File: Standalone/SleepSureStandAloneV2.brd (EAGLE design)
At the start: 62.3 x 37 mm, 79 parts, among them IC1 CP2104, J1 10118192-0002LF, Q1 mmbt2222, Q2 mmbt2222, Q3 DMG3415U, SW2 KMR2, T1 MMUN2133LT1G, U1 ADS1299-4PAG, U2 AP2112-3.3, U3 MCP73831T-2ACI/OT, U4 TPS61090RSAR, X1 JSTPH, X2 ESP32_WROOM32_SKINNY

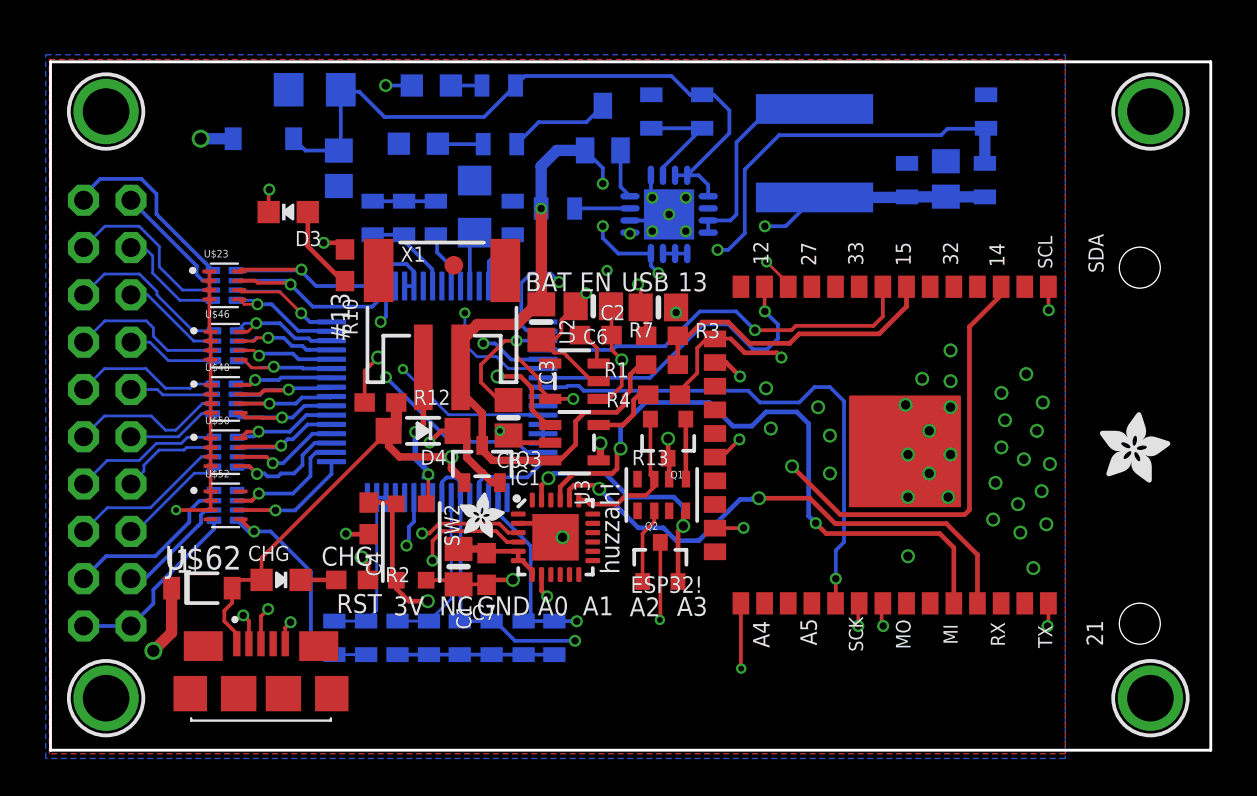
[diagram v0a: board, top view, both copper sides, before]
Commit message: Uploading final standalone and feather files
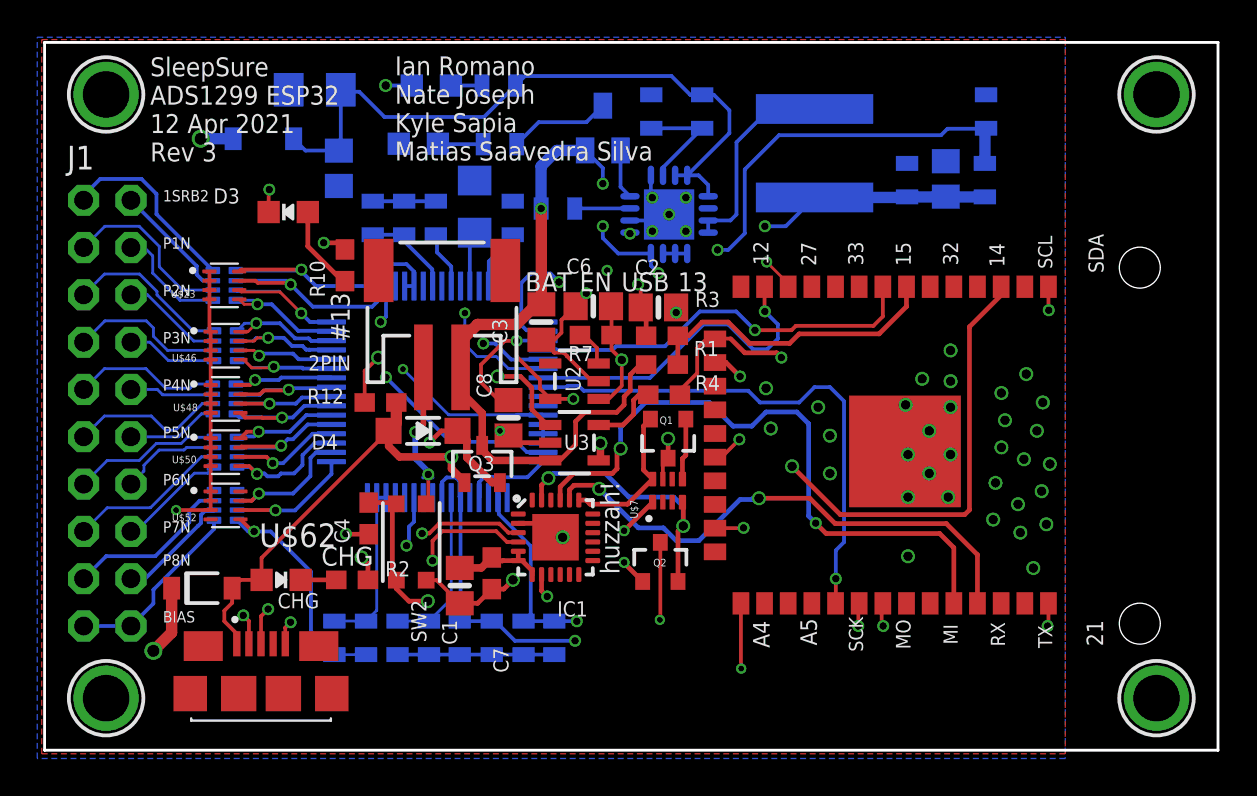
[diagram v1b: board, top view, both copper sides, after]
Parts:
- removed R13: 10K, microbuilder:RESPACK_4X0603
- removed U$14: (no value), microbuilder:ADAFRUIT_2.5MM
- removed U$15: (no value), microbuilder:ADAFRUIT_3.5MM
- removed U$34: FIDUCIAL_1MM, microbuilder:FIDUCIAL_1MM
- added U$7: 10k, SleepSureLib:RESCAXS50P200X100X45-8N
- JP2: value (none) -> 2x10
- U3: value MCP73831T-2ACI/OT -> LiPoly
- moved C1 1.02 mm to (22.3, 8.84)
- moved U$19 0.97 mm to (59.7, 35.2)
- moved U$6 0.92 mm to (3.30, 35.2)
- moved C7 0.36 mm to (24.0, 9.50)
- moved U$31 0.33 mm to (59.7, 2.79)
- renumbered X1 to 2PIN
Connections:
- removed net N$12: Q1.1, R13.5
- removed net N$13: Q2.1, R13.2
- new net N$2: Q2.1, U$7.1
- new net N$6: Q1.1, U$7.5
- net 3.3V: now also U$7.2; no longer R13.3
- net DTR: now also U$7.4; no longer R13.4
- net RESET: now also U$7.7; no longer R13.6
- net RTS: now also U$7.8; no longer R13.7
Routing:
- net N$2: track 0.00 -> 5.30 mm, vias 0 -> 2
- net N$13: track 4.06 -> 0.00 mm
- net N$6: track 0.00 -> 3.30 mm
- net N$12: track 3.23 -> 0.00 mm
- net GND: track 81.5 -> 82.7 mm
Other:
- board size 62.3 x 37 mm -> 63 x 38 mm
- board text added: "1SRB2"
- board text added: "BIAS"
- board text added: "Ian Romano Nate Joseph Kyle Sapia Matias Saavedra Silva"
- board text added: "P1N"
- board text added: "P2N"
- board text added: "P3N"
- board text added: "P4N"
- board text added: "P5N"
- board text added: "P6N"
- board text added: "P7N"
- board text added: "P8N"
- board text added: "SleepSure ADS1299 ESP32 12 Apr 2021 Rev 3"
- board text removed: "3.7/4.2V LiPoly Batt µUSB charge"
- board text removed: "3V"
- board text removed: "A0"
- board text removed: "A1"
- board text removed: "A2"
- board text removed: "A3"
- board text removed: "ESP32 Feather 16MB Flash WiFI+BT"
- board text removed: "ESP32!"
- board text removed: "GND"
- board text removed: "NC"
- board text removed: "RST"
